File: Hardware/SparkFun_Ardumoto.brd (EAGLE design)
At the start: 59.7 x 53.3 mm, 66 parts, among them U1 ARDUINO, U2 L298, U5 74HC1G04, U6 74HC1G04

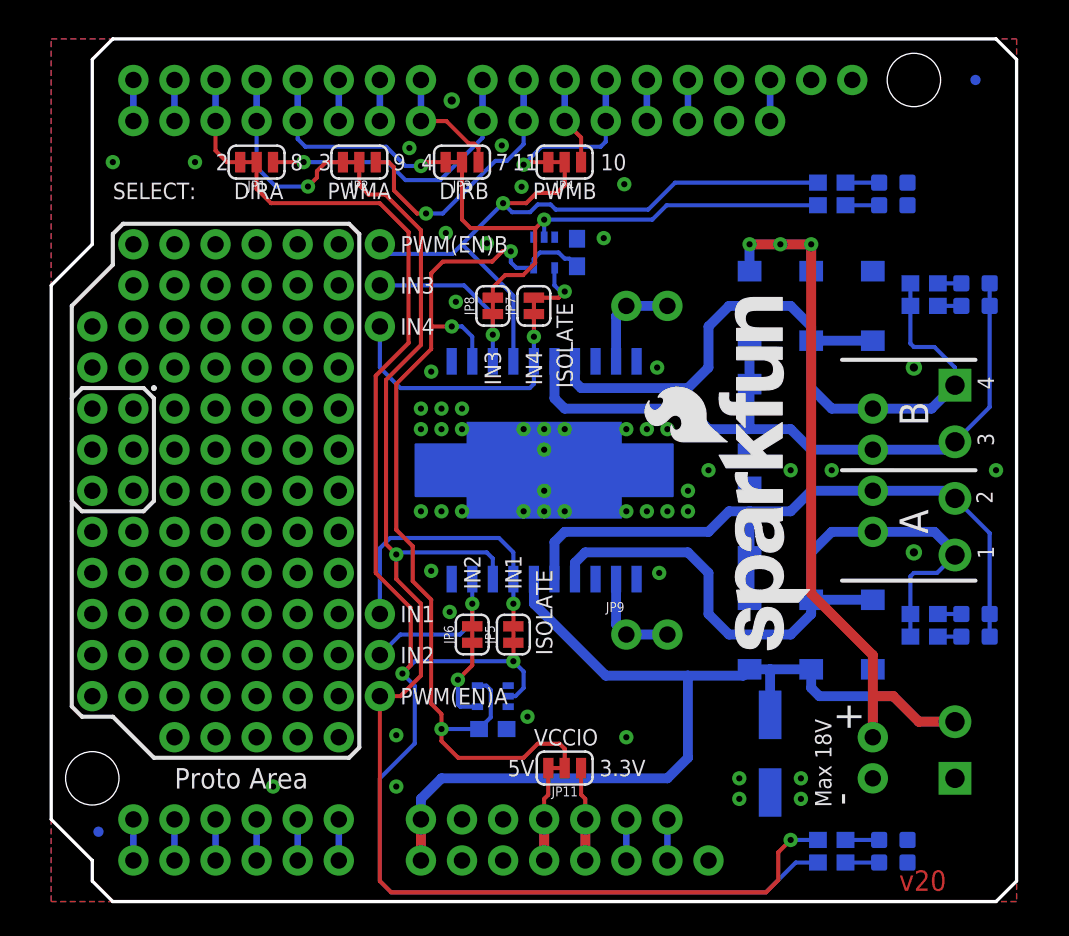
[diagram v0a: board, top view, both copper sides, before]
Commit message: Made post-review changes
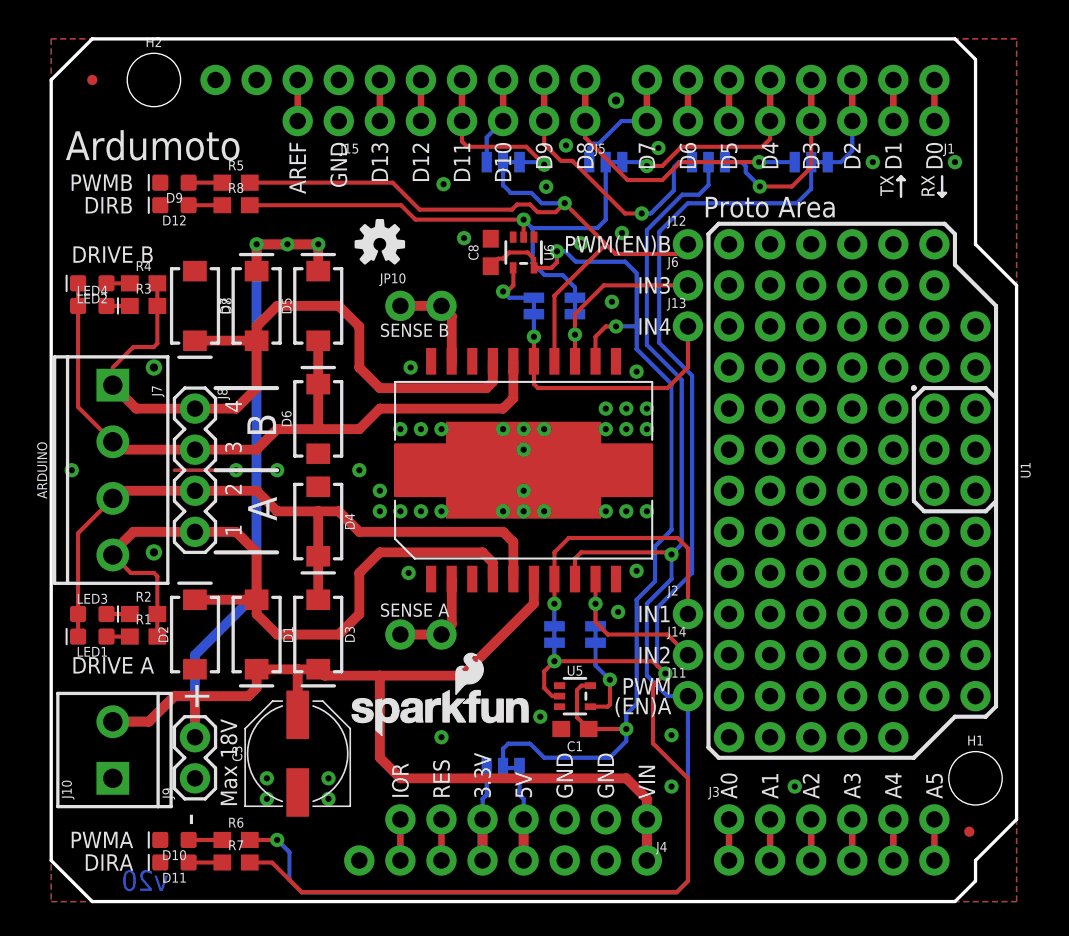
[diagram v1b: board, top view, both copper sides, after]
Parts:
- moved FRAME2 105.4 mm to (-22.9, -11.4), flipped to the top
- moved FRAME1 64.8 mm to (-2.56, -15.2), flipped to the top
- moved FD1 54.6 mm to (2.54, 50.8), flipped to the top
- moved H1 54.6 mm to (57.1, 7.62), flipped to the top
- moved LED1 54.6 mm to (2.54, 16.4), flipped to the top
- moved LED2 54.6 mm to (2.54, 38.2), flipped to the top
- moved LED3 54.6 mm to (2.54, 17.8), flipped to the top
- moved LED4 54.6 mm to (2.54, 36.8), flipped to the top
- moved FD2 53.8 mm to (56.8, 4.32), flipped to the top
- moved J10 52.1 mm to (3.81, 7.62), flipped to the top
- moved J7 52.1 mm to (3.81, 31.9), flipped to the top
- moved J1 49.5 mm to (54.6, 48.3), flipped to the top
- moved R1 48.3 mm to (5.71, 16.4), flipped to the top
- moved R2 48.3 mm to (5.71, 17.8), flipped to the top
- moved R3 48.3 mm to (5.71, 36.8), flipped to the top
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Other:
- outline, holes or cut-outs redrawn
